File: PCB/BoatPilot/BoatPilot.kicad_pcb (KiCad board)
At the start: 4 copper layers, 65 x 35.5 mm, 107 parts, among them J101 battery, J102 Raspberry_Pi_2_3, J103 FlexInput, J104 out 1, J105 SWD, J106 out 2, J107 out 3, J108 UART, J109 out 4, J110 out 5, J111 out 6, J112 GPS, J113 I2C Flex, J114 wind, J115 ANT, J116 USB_OTG, J117 Micro_SD_Card, Q101 TSM3457, U101 TPS565208, U102 TLV75733PDBV, U103 TLV75733PDBV, U104 BMX160, U105 STM32F405RGTx, U106 74LVC1G86, U107 P-SENSE, U108 W25Q128JVS, U109 TLV75733PDBV, U111 RFM69HCW, Y101 8MHz

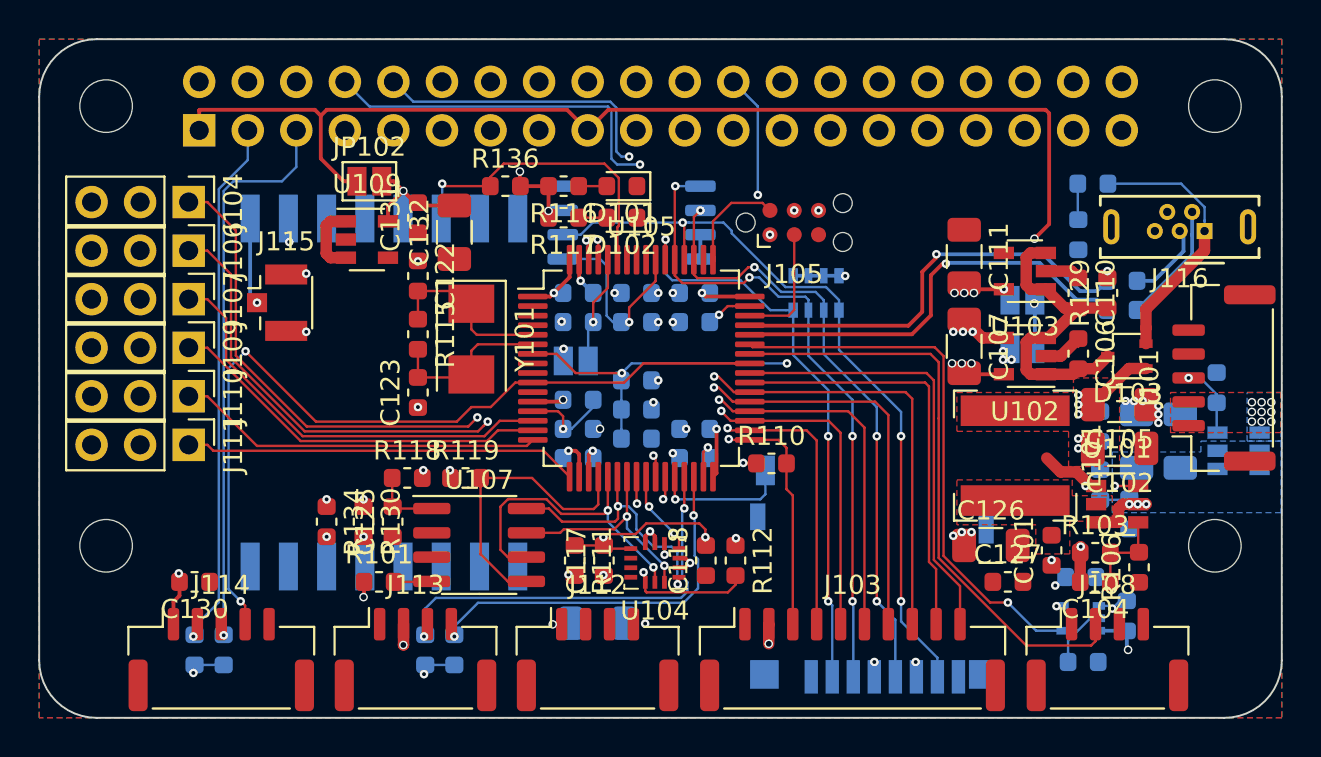
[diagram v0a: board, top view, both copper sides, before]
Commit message: Layout in work
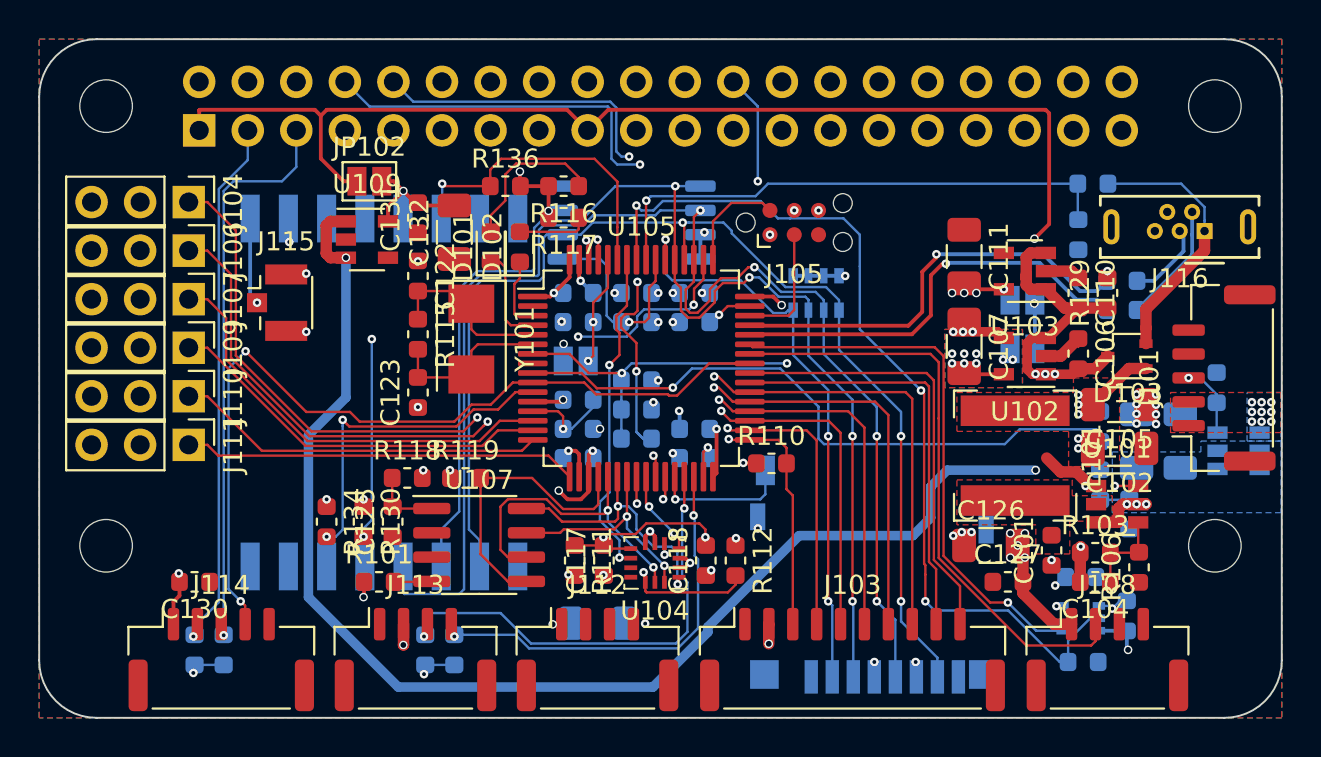
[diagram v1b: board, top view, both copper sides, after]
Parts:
- moved D101 7.56 mm to (36.1, 35.4), turned to 90 degrees
- moved D102 5.55 mm to (37.6, 35.4), turned to 90 degrees
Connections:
- U105 pad 11: (no net) -> /RFM_RST
- U105 pad 3: /LED_WARN -> /LED_STAT
- U105 pad 4: /LED_STAT -> /LED_WARN
- U105 pad 57: /BMX160_INT2 -> /UART_INV
- U105 pad 58: /RFM_RST -> /BMX160_INT2
- U105 pad 8: /UART_INV -> (no net)
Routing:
- net +5V: track 20.7 -> 106.1 mm, vias 0 -> 10
- net /UART_INV: track 3.22 -> 48.2 mm, vias 0 -> 3
- net +3.3VA: track 20.6 -> 65.3 mm
- net /SPI3_SCK: track 32.6 -> 71.8 mm
- net /UBATT: track 1.47 -> 35.4 mm, vias 0 -> 1
- net /SPI3_MOSI: track 34.5 -> 66.9 mm
- net /~CS_RFM69: track 1.58 -> 32.8 mm, vias 1 -> 4
- net /VBUS_SENSE: track 1.89 -> 27.9 mm, vias 0 -> 1
- net /SPI3_MISO: track 40.3 -> 62.2 mm
- net Net-(J102-Pad15): track 0.00 -> 21.9 mm, vias 0 -> 2
- net /RFM_RST: track 1.56 -> 19.1 mm, vias 1 -> 2
- net /BMX160_INT2: track 0.00 -> 17.3 mm, vias 0 -> 2
- net +3V3: track 34.9 -> 44.4 mm, vias 31 -> 36
- net Net-(D101-Pad2): track 1.47 -> 8.15 mm
- net /LED_WARN: track 0.00 -> 5.17 mm
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- added copper zone on B.Cu, net +3V3
- added copper zone on F.Cu, net +3V3
